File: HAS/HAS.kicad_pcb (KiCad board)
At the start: 2 copper layers, 64 x 64 mm, 5 parts

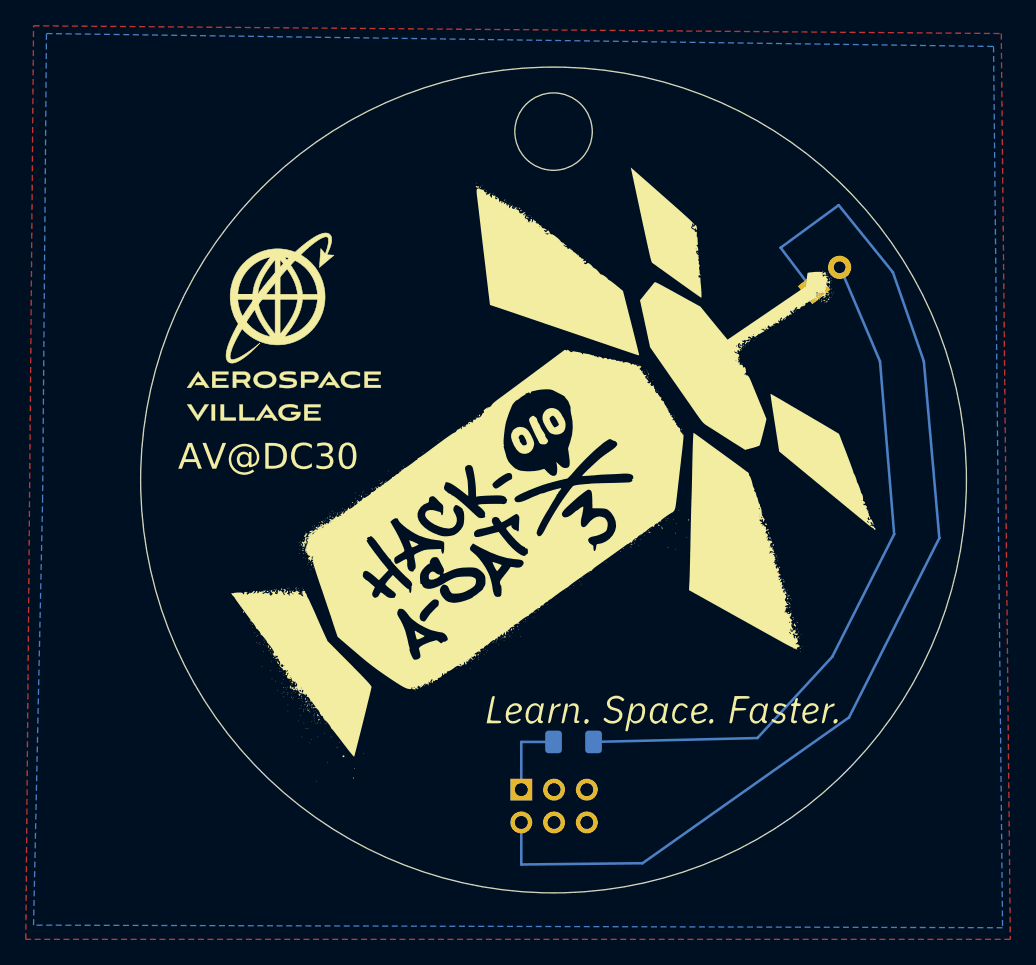
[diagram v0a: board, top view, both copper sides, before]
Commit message: v3 of HAS SAO
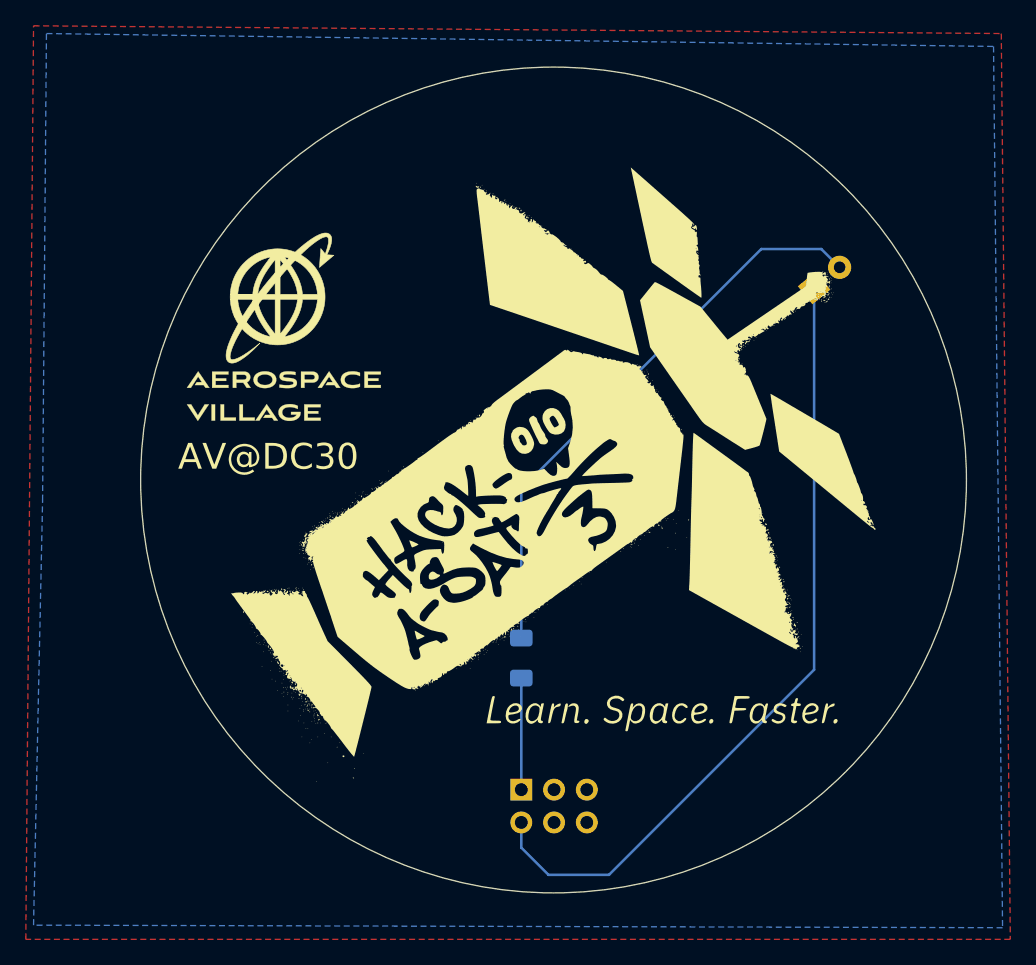
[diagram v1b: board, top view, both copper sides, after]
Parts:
- removed the G*** at (160.0, 100.0)
- moved REF** 7.66 mm to (157.5, 113.8), turned to 90 degrees
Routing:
- net (no net): track 0.00 -> 114.9 mm
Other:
- outline, holes or cut-outs redrawn
- board text added: "v3"
- board text removed: "v2"
